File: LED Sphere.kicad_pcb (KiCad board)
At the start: 2 copper layers, 62 x 45.5 mm, 28 parts, among them J1 Conn_01x03, J2 Conn_01x03

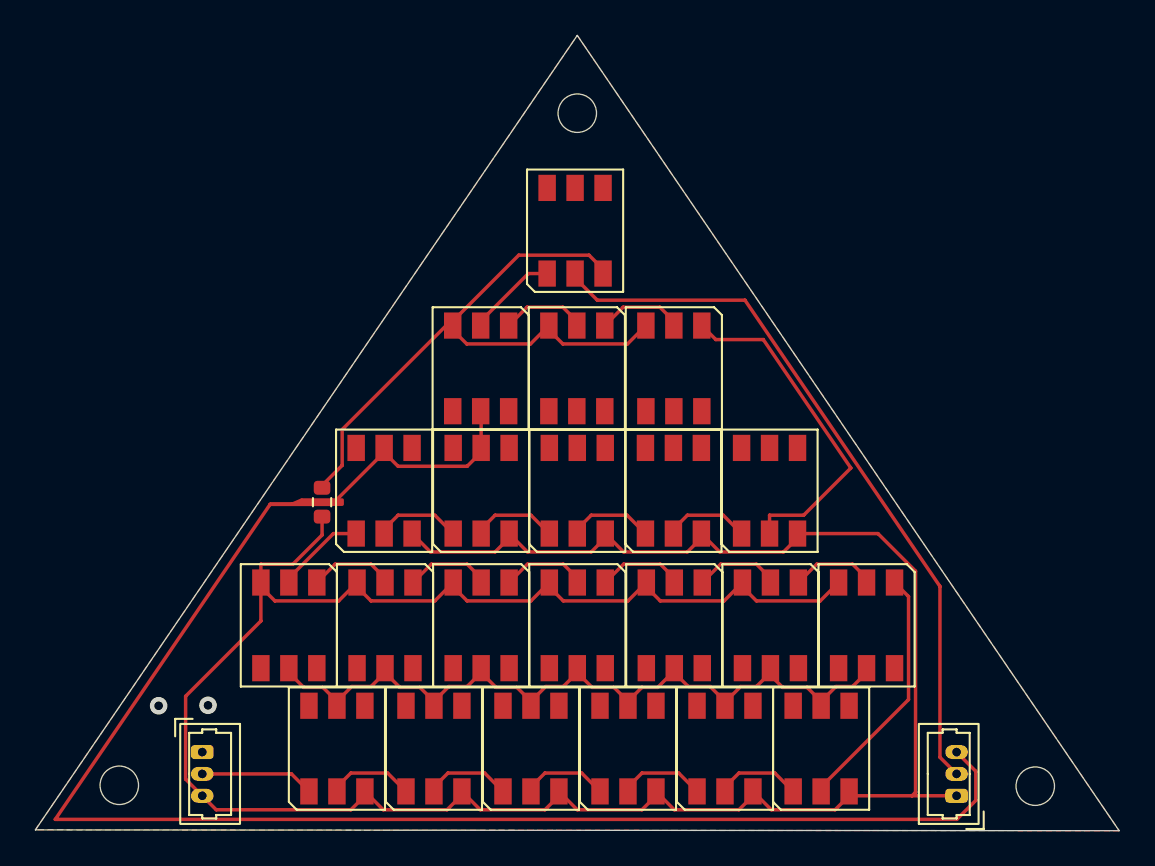
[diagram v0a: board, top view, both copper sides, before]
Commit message: Add files via upload
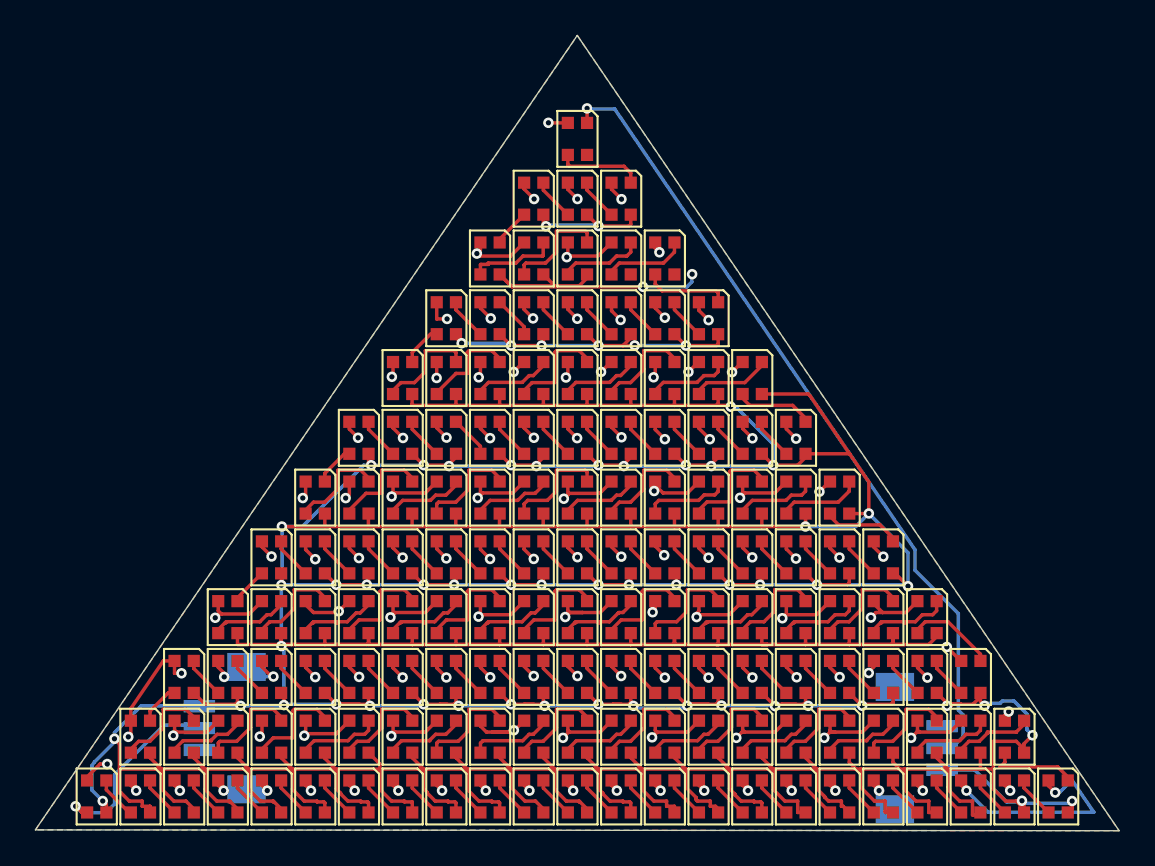
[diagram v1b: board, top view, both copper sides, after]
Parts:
- removed H1, H2, H3: MountingHole, MountingHole:MountingHole_2.2mm_M2
- removed J2: Conn_01x03, Connector_Molex:Molex_PicoBlade_53047-0310_1x03_P1.25mm_Vertical
- removed R1: 0 Ohm, Resistor_SMD:R_0603_1608Metric
- added D100: WS2812B-2020, LED_SMD:LED_WS2812B-2020_PLCC4_2.0x2.0mm, F.Cu at (128.2, 48.6)
- added D101: WS2812B-2020, LED_SMD:LED_WS2812B-2020_PLCC4_2.0x2.0mm, F.Cu at (125.7, 48.6)
- added D102: WS2812B-2020, LED_SMD:LED_WS2812B-2020_PLCC4_2.0x2.0mm, F.Cu at (123.2, 48.6)
- added D103: WS2812B-2020, LED_SMD:LED_WS2812B-2020_PLCC4_2.0x2.0mm, F.Cu at (120.7, 48.6)
- added D104: WS2812B-2020, LED_SMD:LED_WS2812B-2020_PLCC4_2.0x2.0mm, F.Cu at (118.2, 48.6)
- added D105: WS2812B-2020, LED_SMD:LED_WS2812B-2020_PLCC4_2.0x2.0mm, F.Cu at (115.7, 48.6)
- added D106: WS2812B-2020, LED_SMD:LED_WS2812B-2020_PLCC4_2.0x2.0mm, F.Cu at (113.2, 48.6)
- added D107: WS2812B-2020, LED_SMD:LED_WS2812B-2020_PLCC4_2.0x2.0mm, F.Cu at (110.7, 48.6)
- added D108: WS2812B-2020, LED_SMD:LED_WS2812B-2020_PLCC4_2.0x2.0mm, F.Cu at (108.2, 48.6)
- added D109: WS2812B-2020, LED_SMD:LED_WS2812B-2020_PLCC4_2.0x2.0mm, F.Cu at (110.7, 45.2)
- added D110: WS2812B-2020, LED_SMD:LED_WS2812B-2020_PLCC4_2.0x2.0mm, F.Cu at (113.2, 45.2)
- added D111: WS2812B-2020, LED_SMD:LED_WS2812B-2020_PLCC4_2.0x2.0mm, F.Cu at (115.7, 45.2)
- added D112: WS2812B-2020, LED_SMD:LED_WS2812B-2020_PLCC4_2.0x2.0mm, F.Cu at (118.2, 45.2)
- added D113: WS2812B-2020, LED_SMD:LED_WS2812B-2020_PLCC4_2.0x2.0mm, F.Cu at (120.7, 45.2)
- added D114: WS2812B-2020, LED_SMD:LED_WS2812B-2020_PLCC4_2.0x2.0mm, F.Cu at (123.2, 45.2)
- added D115: WS2812B-2020, LED_SMD:LED_WS2812B-2020_PLCC4_2.0x2.0mm, F.Cu at (125.7, 45.2)
- added D116: WS2812B-2020, LED_SMD:LED_WS2812B-2020_PLCC4_2.0x2.0mm, F.Cu at (128.2, 45.2)
- added D117: WS2812B-2020, LED_SMD:LED_WS2812B-2020_PLCC4_2.0x2.0mm, F.Cu at (130.7, 45.2)
- added D118: WS2812B-2020, LED_SMD:LED_WS2812B-2020_PLCC4_2.0x2.0mm, F.Cu at (133.2, 45.2)
- added D119: WS2812B-2020, LED_SMD:LED_WS2812B-2020_PLCC4_2.0x2.0mm, F.Cu at (135.7, 45.2)
- added D120: WS2812B-2020, LED_SMD:LED_WS2812B-2020_PLCC4_2.0x2.0mm, F.Cu at (133.2, 41.8)
- added D121: WS2812B-2020, LED_SMD:LED_WS2812B-2020_PLCC4_2.0x2.0mm, F.Cu at (130.7, 41.8)
- added D122: WS2812B-2020, LED_SMD:LED_WS2812B-2020_PLCC4_2.0x2.0mm, F.Cu at (128.2, 41.8)
- added D123: WS2812B-2020, LED_SMD:LED_WS2812B-2020_PLCC4_2.0x2.0mm, F.Cu at (125.7, 41.8)
- added D124: WS2812B-2020, LED_SMD:LED_WS2812B-2020_PLCC4_2.0x2.0mm, F.Cu at (123.2, 41.8)
- added D125: WS2812B-2020, LED_SMD:LED_WS2812B-2020_PLCC4_2.0x2.0mm, F.Cu at (120.7, 41.8)
- added D126: WS2812B-2020, LED_SMD:LED_WS2812B-2020_PLCC4_2.0x2.0mm, F.Cu at (118.2, 41.8)
- added D127: WS2812B-2020, LED_SMD:LED_WS2812B-2020_PLCC4_2.0x2.0mm, F.Cu at (115.7, 41.8)
- added D128: WS2812B-2020, LED_SMD:LED_WS2812B-2020_PLCC4_2.0x2.0mm, F.Cu at (113.2, 41.8)
- added D129: WS2812B-2020, LED_SMD:LED_WS2812B-2020_PLCC4_2.0x2.0mm, F.Cu at (115.7, 38.3)
- added D130: WS2812B-2020, LED_SMD:LED_WS2812B-2020_PLCC4_2.0x2.0mm, F.Cu at (118.2, 38.3)
- added D131: WS2812B-2020, LED_SMD:LED_WS2812B-2020_PLCC4_2.0x2.0mm, F.Cu at (120.7, 38.3)
- added D132: WS2812B-2020, LED_SMD:LED_WS2812B-2020_PLCC4_2.0x2.0mm, F.Cu at (123.2, 38.3)
- added D133: WS2812B-2020, LED_SMD:LED_WS2812B-2020_PLCC4_2.0x2.0mm, F.Cu at (125.7, 38.3)
- added D134: WS2812B-2020, LED_SMD:LED_WS2812B-2020_PLCC4_2.0x2.0mm, F.Cu at (128.2, 38.3)
- added D135: WS2812B-2020, LED_SMD:LED_WS2812B-2020_PLCC4_2.0x2.0mm, F.Cu at (130.7, 38.3)
- added D136: WS2812B-2020, LED_SMD:LED_WS2812B-2020_PLCC4_2.0x2.0mm, F.Cu at (128.2, 34.9)
- added D137: WS2812B-2020, LED_SMD:LED_WS2812B-2020_PLCC4_2.0x2.0mm, F.Cu at (125.7, 34.9)
- added D138: WS2812B-2020, LED_SMD:LED_WS2812B-2020_PLCC4_2.0x2.0mm, F.Cu at (123.2, 34.9)
- added D139: WS2812B-2020, LED_SMD:LED_WS2812B-2020_PLCC4_2.0x2.0mm, F.Cu at (120.7, 34.9)
- added D140: WS2812B-2020, LED_SMD:LED_WS2812B-2020_PLCC4_2.0x2.0mm, F.Cu at (118.2, 34.9)
- added D141: WS2812B-2020, LED_SMD:LED_WS2812B-2020_PLCC4_2.0x2.0mm, F.Cu at (120.7, 31.5)
- added D142: WS2812B-2020, LED_SMD:LED_WS2812B-2020_PLCC4_2.0x2.0mm, F.Cu at (123.2, 31.5)
- added D143: WS2812B-2020, LED_SMD:LED_WS2812B-2020_PLCC4_2.0x2.0mm, F.Cu at (125.7, 31.5)
- added D144: WS2812B-2020, LED_SMD:LED_WS2812B-2020_PLCC4_2.0x2.0mm, F.Cu at (123.2, 28.1)
- added D23: WS2812B-2020, LED_SMD:LED_WS2812B-2020_PLCC4_2.0x2.0mm, F.Cu at (150.7, 65.7)
- added D24: WS2812B-2020, LED_SMD:LED_WS2812B-2020_PLCC4_2.0x2.0mm, F.Cu at (148.2, 62.3)
- added D25: WS2812B-2020, LED_SMD:LED_WS2812B-2020_PLCC4_2.0x2.0mm, F.Cu at (145.7, 62.3)
- added D26: WS2812B-2020, LED_SMD:LED_WS2812B-2020_PLCC4_2.0x2.0mm, F.Cu at (143.2, 62.3)
- added D27: WS2812B-2020, LED_SMD:LED_WS2812B-2020_PLCC4_2.0x2.0mm, F.Cu at (140.7, 62.3)
- added D28: WS2812B-2020, LED_SMD:LED_WS2812B-2020_PLCC4_2.0x2.0mm, F.Cu at (138.2, 62.3)
- added D29: WS2812B-2020, LED_SMD:LED_WS2812B-2020_PLCC4_2.0x2.0mm, F.Cu at (135.7, 62.3)
- added D30: WS2812B-2020, LED_SMD:LED_WS2812B-2020_PLCC4_2.0x2.0mm, F.Cu at (133.2, 62.3)
- added D31: WS2812B-2020, LED_SMD:LED_WS2812B-2020_PLCC4_2.0x2.0mm, F.Cu at (130.7, 62.3)
- added D32: WS2812B-2020, LED_SMD:LED_WS2812B-2020_PLCC4_2.0x2.0mm, F.Cu at (128.2, 62.3)
- added D33: WS2812B-2020, LED_SMD:LED_WS2812B-2020_PLCC4_2.0x2.0mm, F.Cu at (125.7, 62.3)
- added D34: WS2812B-2020, LED_SMD:LED_WS2812B-2020_PLCC4_2.0x2.0mm, F.Cu at (123.2, 62.3)
- added D35: WS2812B-2020, LED_SMD:LED_WS2812B-2020_PLCC4_2.0x2.0mm, F.Cu at (120.7, 62.3)
- added D36: WS2812B-2020, LED_SMD:LED_WS2812B-2020_PLCC4_2.0x2.0mm, F.Cu at (118.2, 62.3)
- added D37: WS2812B-2020, LED_SMD:LED_WS2812B-2020_PLCC4_2.0x2.0mm, F.Cu at (115.7, 62.3)
- added D38: WS2812B-2020, LED_SMD:LED_WS2812B-2020_PLCC4_2.0x2.0mm, F.Cu at (113.2, 62.3)
- added D39: WS2812B-2020, LED_SMD:LED_WS2812B-2020_PLCC4_2.0x2.0mm, F.Cu at (110.7, 62.3)
- added D40: WS2812B-2020, LED_SMD:LED_WS2812B-2020_PLCC4_2.0x2.0mm, F.Cu at (108.2, 62.3)
- added D41: WS2812B-2020, LED_SMD:LED_WS2812B-2020_PLCC4_2.0x2.0mm, F.Cu at (105.7, 62.3)
- added D42: WS2812B-2020, LED_SMD:LED_WS2812B-2020_PLCC4_2.0x2.0mm, F.Cu at (103.2, 62.3)
- added D43: WS2812B-2020, LED_SMD:LED_WS2812B-2020_PLCC4_2.0x2.0mm, F.Cu at (100.7, 62.3)
- added D44: WS2812B-2020, LED_SMD:LED_WS2812B-2020_PLCC4_2.0x2.0mm, F.Cu at (98.2, 62.3)
- added D45: WS2812B-2020, LED_SMD:LED_WS2812B-2020_PLCC4_2.0x2.0mm, F.Cu at (100.7, 58.9)
- added D46: WS2812B-2020, LED_SMD:LED_WS2812B-2020_PLCC4_2.0x2.0mm, F.Cu at (103.2, 58.9)
- added D47: WS2812B-2020, LED_SMD:LED_WS2812B-2020_PLCC4_2.0x2.0mm, F.Cu at (105.7, 58.9)
- added D48: WS2812B-2020, LED_SMD:LED_WS2812B-2020_PLCC4_2.0x2.0mm, F.Cu at (108.2, 58.9)
- added D49: WS2812B-2020, LED_SMD:LED_WS2812B-2020_PLCC4_2.0x2.0mm, F.Cu at (110.7, 58.9)
- added D50: WS2812B-2020, LED_SMD:LED_WS2812B-2020_PLCC4_2.0x2.0mm, F.Cu at (113.2, 58.9)
- added D51: WS2812B-2020, LED_SMD:LED_WS2812B-2020_PLCC4_2.0x2.0mm, F.Cu at (115.7, 58.9)
- added D52: WS2812B-2020, LED_SMD:LED_WS2812B-2020_PLCC4_2.0x2.0mm, F.Cu at (118.2, 58.9)
- added D53: WS2812B-2020, LED_SMD:LED_WS2812B-2020_PLCC4_2.0x2.0mm, F.Cu at (120.7, 58.9)
- added D54: WS2812B-2020, LED_SMD:LED_WS2812B-2020_PLCC4_2.0x2.0mm, F.Cu at (123.2, 58.9)
- added D55: WS2812B-2020, LED_SMD:LED_WS2812B-2020_PLCC4_2.0x2.0mm, F.Cu at (125.7, 58.9)
- added D56: WS2812B-2020, LED_SMD:LED_WS2812B-2020_PLCC4_2.0x2.0mm, F.Cu at (128.2, 58.9)
- added D57: WS2812B-2020, LED_SMD:LED_WS2812B-2020_PLCC4_2.0x2.0mm, F.Cu at (130.7, 58.9)
- added D58: WS2812B-2020, LED_SMD:LED_WS2812B-2020_PLCC4_2.0x2.0mm, F.Cu at (133.2, 58.9)
- added D59: WS2812B-2020, LED_SMD:LED_WS2812B-2020_PLCC4_2.0x2.0mm, F.Cu at (135.7, 58.9)
- added D60: WS2812B-2020, LED_SMD:LED_WS2812B-2020_PLCC4_2.0x2.0mm, F.Cu at (138.2, 58.9)
- added D61: WS2812B-2020, LED_SMD:LED_WS2812B-2020_PLCC4_2.0x2.0mm, F.Cu at (140.7, 58.9)
- added D62: WS2812B-2020, LED_SMD:LED_WS2812B-2020_PLCC4_2.0x2.0mm, F.Cu at (143.2, 58.9)
- added D63: WS2812B-2020, LED_SMD:LED_WS2812B-2020_PLCC4_2.0x2.0mm, F.Cu at (145.7, 58.9)
- added D64: WS2812B-2020, LED_SMD:LED_WS2812B-2020_PLCC4_2.0x2.0mm, F.Cu at (143.2, 55.4)
- added D65: WS2812B-2020, LED_SMD:LED_WS2812B-2020_PLCC4_2.0x2.0mm, F.Cu at (140.7, 55.4)
- added D66: WS2812B-2020, LED_SMD:LED_WS2812B-2020_PLCC4_2.0x2.0mm, F.Cu at (138.2, 55.4)
- added D67: WS2812B-2020, LED_SMD:LED_WS2812B-2020_PLCC4_2.0x2.0mm, F.Cu at (135.7, 55.4)
- added D68: WS2812B-2020, LED_SMD:LED_WS2812B-2020_PLCC4_2.0x2.0mm, F.Cu at (133.2, 55.4)
- added D69: WS2812B-2020, LED_SMD:LED_WS2812B-2020_PLCC4_2.0x2.0mm, F.Cu at (130.7, 55.4)
- added D70: WS2812B-2020, LED_SMD:LED_WS2812B-2020_PLCC4_2.0x2.0mm, F.Cu at (128.2, 55.4)
- added D71: WS2812B-2020, LED_SMD:LED_WS2812B-2020_PLCC4_2.0x2.0mm, F.Cu at (125.7, 55.4)
- added D72: WS2812B-2020, LED_SMD:LED_WS2812B-2020_PLCC4_2.0x2.0mm, F.Cu at (123.2, 55.4)
- added D73: WS2812B-2020, LED_SMD:LED_WS2812B-2020_PLCC4_2.0x2.0mm, F.Cu at (120.7, 55.4)
- added D74: WS2812B-2020, LED_SMD:LED_WS2812B-2020_PLCC4_2.0x2.0mm, F.Cu at (118.2, 55.4)
- added D75: WS2812B-2020, LED_SMD:LED_WS2812B-2020_PLCC4_2.0x2.0mm, F.Cu at (115.7, 55.4)
- added D76: WS2812B-2020, LED_SMD:LED_WS2812B-2020_PLCC4_2.0x2.0mm, F.Cu at (113.2, 55.4)
- added D77: WS2812B-2020, LED_SMD:LED_WS2812B-2020_PLCC4_2.0x2.0mm, F.Cu at (110.7, 55.4)
- added D78: WS2812B-2020, LED_SMD:LED_WS2812B-2020_PLCC4_2.0x2.0mm, F.Cu at (108.2, 55.4)
- added D79: WS2812B-2020, LED_SMD:LED_WS2812B-2020_PLCC4_2.0x2.0mm, F.Cu at (105.7, 55.4)
- added D80: WS2812B-2020, LED_SMD:LED_WS2812B-2020_PLCC4_2.0x2.0mm, F.Cu at (103.2, 55.4)
- added D81: WS2812B-2020, LED_SMD:LED_WS2812B-2020_PLCC4_2.0x2.0mm, F.Cu at (105.7, 52.0)
- added D82: WS2812B-2020, LED_SMD:LED_WS2812B-2020_PLCC4_2.0x2.0mm, F.Cu at (108.2, 52.0)
- added D83: WS2812B-2020, LED_SMD:LED_WS2812B-2020_PLCC4_2.0x2.0mm, F.Cu at (110.7, 52.0)
- added D84: WS2812B-2020, LED_SMD:LED_WS2812B-2020_PLCC4_2.0x2.0mm, F.Cu at (113.2, 52.0)
- added D85: WS2812B-2020, LED_SMD:LED_WS2812B-2020_PLCC4_2.0x2.0mm, F.Cu at (115.7, 52.0)
- added D86: WS2812B-2020, LED_SMD:LED_WS2812B-2020_PLCC4_2.0x2.0mm, F.Cu at (118.2, 52.0)
- added D87: WS2812B-2020, LED_SMD:LED_WS2812B-2020_PLCC4_2.0x2.0mm, F.Cu at (120.7, 52.0)
- added D88: WS2812B-2020, LED_SMD:LED_WS2812B-2020_PLCC4_2.0x2.0mm, F.Cu at (123.2, 52.0)
- added D89: WS2812B-2020, LED_SMD:LED_WS2812B-2020_PLCC4_2.0x2.0mm, F.Cu at (125.7, 52.0)
- added D90: WS2812B-2020, LED_SMD:LED_WS2812B-2020_PLCC4_2.0x2.0mm, F.Cu at (128.2, 52.0)
- added D91: WS2812B-2020, LED_SMD:LED_WS2812B-2020_PLCC4_2.0x2.0mm, F.Cu at (130.7, 52.0)
- added D92: WS2812B-2020, LED_SMD:LED_WS2812B-2020_PLCC4_2.0x2.0mm, F.Cu at (133.2, 52.0)
- added D93: WS2812B-2020, LED_SMD:LED_WS2812B-2020_PLCC4_2.0x2.0mm, F.Cu at (135.7, 52.0)
- added D94: WS2812B-2020, LED_SMD:LED_WS2812B-2020_PLCC4_2.0x2.0mm, F.Cu at (138.2, 52.0)
- added D95: WS2812B-2020, LED_SMD:LED_WS2812B-2020_PLCC4_2.0x2.0mm, F.Cu at (140.7, 52.0)
- added D96: WS2812B-2020, LED_SMD:LED_WS2812B-2020_PLCC4_2.0x2.0mm, F.Cu at (138.2, 48.6)
- added D97: WS2812B-2020, LED_SMD:LED_WS2812B-2020_PLCC4_2.0x2.0mm, F.Cu at (135.7, 48.6)
- added D98: WS2812B-2020, LED_SMD:LED_WS2812B-2020_PLCC4_2.0x2.0mm, F.Cu at (133.2, 48.6)
- added D99: WS2812B-2020, LED_SMD:LED_WS2812B-2020_PLCC4_2.0x2.0mm, F.Cu at (130.7, 48.6)
- added J3: Conn_01x03_MountingPin, Connector_Hirose:Hirose_DF13C_CL535-0403-5-51_1x03-1MP_P1.25mm_Vertical, B.Cu at (103.0, 61.8)
- D1, D10, D11, D12, D13, D14, D15, D16, D17, D18, D19, D2, D20, D21, D22, D3, D4, D5, D6, D7, D8, D9: value WS2812 -> WS2812B-2020; footprint LED_SMD:LED_WS2812_PLCC6_5.0x5.0mm_P1.6mm -> LED_SMD:LED_WS2812B-2020_PLCC4_2.0x2.0mm
- J1: value Conn_01x03 -> Conn_01x03_MountingPin; footprint Connector_Molex:Molex_PicoBlade_53047-0310_1x03_P1.25mm_Vertical -> Connector_Hirose:Hirose_DF13C_CL535-0403-5-51_1x03-1MP_P1.25mm_Vertical; moved to B.Cu
- moved D22 41.0 mm to (148.2, 65.7), turned to -90 degrees
- moved J1 40.9 mm to (142.6, 62.9), turned to 90 degrees
- moved D21 37.2 mm to (145.7, 65.7)
- moved D20 31.6 mm to (143.2, 65.7)
- moved D7 30.6 mm to (110.7, 65.7)
- moved D6 29.1 mm to (108.2, 65.7), turned to -90 degrees
- moved D19 27.3 mm to (140.7, 65.7)
- moved D5 26.1 mm to (105.7, 65.7), turned to -90 degrees
- moved D14 23.7 mm to (128.2, 65.7), turned to -90 degrees
- moved D8 23.2 mm to (113.2, 65.7)
- moved D4 23.1 mm to (103.2, 65.7), turned to -90 degrees
- moved D15 21.8 mm to (130.7, 65.7), turned to -90 degrees
- moved D13 21.4 mm to (125.7, 65.7)
- moved D16 20.2 mm to (133.2, 65.7), turned to -90 degrees
- moved D3 20.0 mm to (100.7, 65.7), turned to -90 degrees
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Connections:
- D1 pad 1: /DATA_IN -> Net-(D1-DOUT)
- D1 pad 2: Net-(D1-DIN) -> +5V
- D1 pad 3: +5V -> /DATA_IN
- D1 pad 4: unconnected-(D1-NC-Pad4) -> GND
- D10 pad 2: Net-(D10-DIN) -> +5V
- D10 pad 3: +5V -> Net-(D10-DIN)
- D10 pad 4: unconnected-(D10-NC-Pad4) -> GND
- D11 pad 1: Net-(D10-DIN) -> Net-(D11-DOUT)
- D11 pad 2: Net-(D11-DIN) -> +5V
- D11 pad 3: +5V -> Net-(D10-DOUT)
- D11 pad 4: unconnected-(D11-NC-Pad4) -> GND
- D12 pad 1: Net-(D11-DIN) -> Net-(D12-DOUT)
- D12 pad 2: Net-(D12-DIN) -> +5V
- D12 pad 3: +5V -> Net-(D11-DOUT)
- D12 pad 4: unconnected-(D12-NC-Pad4) -> GND
- D13 pad 1: Net-(D12-DIN) -> Net-(D13-DOUT)
- D13 pad 2: Net-(D13-DIN) -> +5V
- D13 pad 3: +5V -> Net-(D12-DOUT)
- D13 pad 4: unconnected-(D13-NC-Pad4) -> GND
- D14 pad 1: Net-(D13-DIN) -> Net-(D14-DOUT)
- D14 pad 2: Net-(D14-DIN) -> +5V
- D14 pad 3: +5V -> Net-(D13-DOUT)
- D14 pad 4: unconnected-(D14-NC-Pad4) -> GND
- D15 pad 1: Net-(D14-DIN) -> Net-(D15-DOUT)
- D15 pad 2: Net-(D15-DIN) -> +5V
- D15 pad 3: +5V -> Net-(D14-DOUT)
- D15 pad 4: unconnected-(D15-NC-Pad4) -> GND
- D16 pad 1: Net-(D15-DIN) -> Net-(D16-DOUT)
- D16 pad 2: Net-(D16-DIN) -> +5V
- D16 pad 3: +5V -> Net-(D15-DOUT)
- D16 pad 4: unconnected-(D16-NC-Pad4) -> GND
- D17 pad 1: Net-(D16-DIN) -> Net-(D17-DOUT)
- D17 pad 2: Net-(D17-DIN) -> +5V
- D17 pad 3: +5V -> Net-(D16-DOUT)
- D17 pad 4: unconnected-(D17-NC-Pad4) -> GND
- D18 pad 1: Net-(D17-DIN) -> Net-(D18-DOUT)
- D18 pad 2: Net-(D18-DIN) -> +5V
- D18 pad 3: +5V -> Net-(D17-DOUT)
- D18 pad 4: unconnected-(D18-NC-Pad4) -> GND
- D19 pad 1: Net-(D18-DIN) -> Net-(D19-DOUT)
- D19 pad 2: Net-(D19-DIN) -> +5V
- D19 pad 3: +5V -> Net-(D18-DOUT)
- D19 pad 4: unconnected-(D19-NC-Pad4) -> GND
- D2 pad 1: Net-(D1-DIN) -> Net-(D2-DOUT)
- D2 pad 2: Net-(D2-DIN) -> +5V
- D2 pad 3: +5V -> Net-(D1-DOUT)
- D2 pad 4: unconnected-(D2-NC-Pad4) -> GND
- D20 pad 1: Net-(D19-DIN) -> Net-(D20-DOUT)
- D20 pad 2: Net-(D20-DIN) -> +5V
- D20 pad 3: +5V -> Net-(D19-DOUT)
- D20 pad 4: unconnected-(D20-NC-Pad4) -> GND
- D21 pad 1: Net-(D20-DIN) -> Net-(D21-DOUT)
- D21 pad 2: Net-(D21-DIN) -> +5V
- D21 pad 3: +5V -> Net-(D20-DOUT)
- D21 pad 4: unconnected-(D21-NC-Pad4) -> GND
- D22 pad 1: Net-(D21-DIN) -> Net-(D22-DOUT)
- D22 pad 2: /DATA_OUT -> +5V
- D22 pad 3: +5V -> Net-(D21-DOUT)
- D22 pad 4: unconnected-(D22-NC-Pad4) -> GND
- D3 pad 1: Net-(D2-DIN) -> Net-(D3-DOUT)
- D3 pad 2: Net-(D3-DIN) -> +5V
- D3 pad 3: +5V -> Net-(D2-DOUT)
- D3 pad 4: unconnected-(D3-NC-Pad4) -> GND
- D4 pad 1: Net-(D3-DIN) -> Net-(D4-DOUT)
- D4 pad 2: Net-(D4-DIN) -> +5V
- D4 pad 3: +5V -> Net-(D3-DOUT)
- D4 pad 4: unconnected-(D4-NC-Pad4) -> GND
- D5 pad 1: Net-(D4-DIN) -> Net-(D5-DOUT)
- D5 pad 2: Net-(D5-DIN) -> +5V
- D5 pad 3: +5V -> Net-(D4-DOUT)
- D5 pad 4: unconnected-(D5-NC-Pad4) -> GND
- D6 pad 1: Net-(D5-DIN) -> Net-(D6-DOUT)
- D6 pad 2: Net-(D6-DIN) -> +5V
- D6 pad 3: +5V -> Net-(D5-DOUT)
- D6 pad 4: unconnected-(D6-NC-Pad4) -> GND
- D7 pad 1: Net-(D6-DIN) -> Net-(D7-DOUT)
- D7 pad 2: Net-(D7-DIN) -> +5V
- D7 pad 3: +5V -> Net-(D6-DOUT)
- D7 pad 4: unconnected-(D7-NC-Pad4) -> GND
- D8 pad 1: Net-(D7-DIN) -> Net-(D8-DOUT)
- D8 pad 2: Net-(D8-DIN) -> +5V
- D8 pad 3: +5V -> Net-(D7-DOUT)
- D8 pad 4: unconnected-(D8-NC-Pad4) -> GND
- D9 pad 1: Net-(D8-DIN) -> Net-(D10-DIN)
- D9 pad 2: Net-(D10-DOUT) -> +5V
- D9 pad 3: +5V -> Net-(D8-DOUT)
- D9 pad 4: unconnected-(D9-NC-Pad4) -> GND
- J1 pad 2: /DATA_IN -> /DATA_OUT
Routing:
- net GND: track 141.2 -> 579.2 mm, vias 2 -> 61
- net Net-(D18-DIN): track 19.6 -> 0.00 mm
- net +5V: track 193.7 -> 209.3 mm, vias 0 -> 120
- net Net-(D6-DIN): track 14.4 -> 0.00 mm
- net Net-(D102-DOUT): track 0.00 -> 6.25 mm
- net Net-(D138-DOUT): track 0.00 -> 6.25 mm
- net Net-(D124-DOUT): track 0.00 -> 6.15 mm
- net Net-(D98-DOUT): track 0.00 -> 6.14 mm
- net Net-(D76-DOUT): track 0.00 -> 6.09 mm
- net Net-(D74-DOUT): track 0.00 -> 6.09 mm
- net Net-(D72-DOUT): track 0.00 -> 6.09 mm
- net Net-(D70-DOUT): track 0.00 -> 6.09 mm
- net Net-(D36-DOUT): track 0.00 -> 6.04 mm
- net Net-(D127-DOUT): track 0.00 -> 6.04 mm
- net Net-(D69-DOUT): track 0.00 -> 6.04 mm
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- added copper zone on B.Cu, net +5V
